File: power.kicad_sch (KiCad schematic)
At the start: 10 parts, among them U19 SN74ALS04 (КР1533ЛН1), U21 SN74ALS14 (КР1533ТЛ2), U39 IN74ALS32N (КР1533ЛЛ1), U40 IN74ALS00N (КР1533ЛА3), U75 IN74ALS32N (КР1533ЛЛ1)

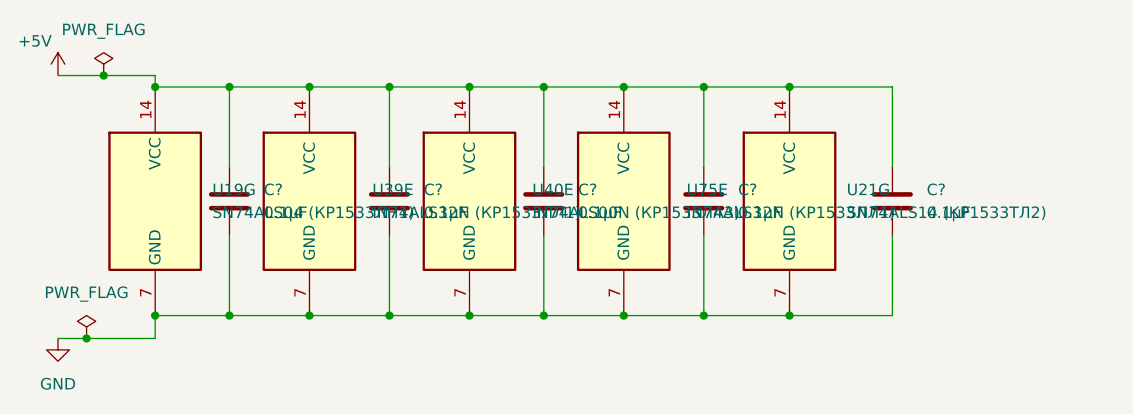
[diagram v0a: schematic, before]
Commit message: March 22nd additions
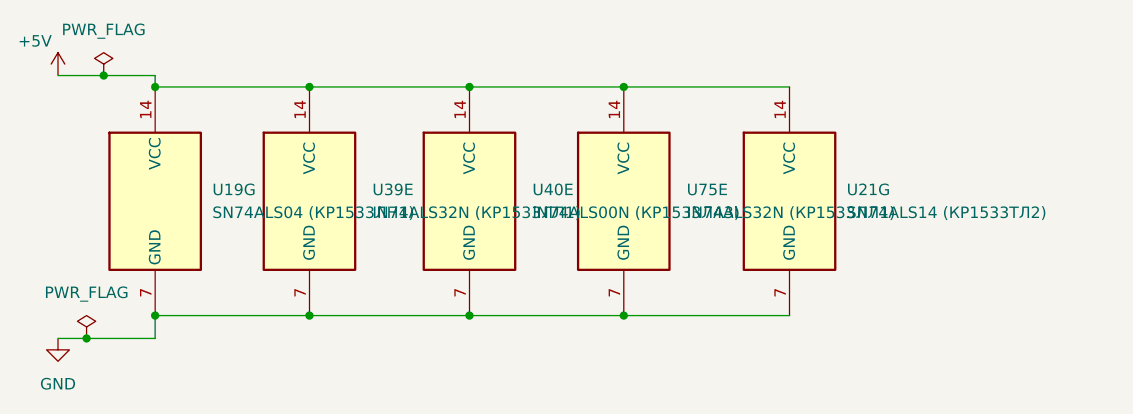
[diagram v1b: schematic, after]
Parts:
- removed C? (x5): 0.1µF, Capacitor_SMD:C_0805_2012Metric, symbol Device:C
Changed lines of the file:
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@@
     (comment 2 "Евстафьев")
   )
-  (junction (at 80.645 54.61) (diameter 0) (color 0 0 0 0)
-  )
-  (junction (at 98.425 54.61) (diameter 0) (color 0 0 0 0)
-  )
-  (junction (at 45.72 29.21) (diameter 0) (color 0 0 0 0)
-  )
   (junction (at 72.39 54.61) (diameter 0) (color 0 0 0 0)
   )
   (junction (at 37.465 29.21) (diameter 0) (color 0 0 0 0)
   )
-  (junction (at 45.72 54.61) (diameter 0) (color 0 0 0 0)
-  )
-  (junction (at 107.95 54.61) (diameter 0) (color 0 0 0 0)
-  )
   (junction (at 29.845 57.15) (diameter 0) (color 0 0 0 0)
   )
@@
   (junction (at 54.61 29.21) (diameter 0) (color 0 0 0 0)
   )
-  (junction (at 98.425 29.21) (diameter 0) (color 0 0 0 0)
-  )
-  (junction (at 107.95 29.21) (diameter 0) (color 0 0 0 0)
-  )
   (junction (at 31.75 27.94) (diameter 0) (color 0 0 0 0)
   )
-  (junction (at 63.5 54.61) (diameter 0) (color 0 0 0 0)
-  )
   (junction (at 72.39 29.21) (diameter 0) (color 0 0 0 0)
   )
-  (junction (at 63.5 29.21) (diameter 0) (color 0 0 0 0)
-  )
-  (junction (at 80.645 29.21) (diameter 0) (color 0 0 0 0)
-  )
   (junction (at 89.535 29.21) (diameter 0) (color 0 0 0 0)
   )
   (junction (at 37.465 54.61) (diameter 0) (color 0 0 0 0)
   )
-  (wire (pts (xy 98.425 29.21) (xy 107.95 29.21))
-    (stroke (width 0) (type default) (color 0 0 0 0))
-  )
-  (wire (pts (xy 119.38 45.72) (xy 119.38 54.61))
-    (stroke (width 0) (type default) (color 0 0 0 0))
-  )
-  (wire (pts (xy 119.38 38.1) (xy 119.38 29.21))
-    (stroke (width 0) (type default) (color 0 0 0 0))
-  )
-  (wire (pts (xy 98.425 54.61) (xy 89.535 54.61))
-    (stroke (width 0) (type default) (color 0 0 0 0))
-  )
-  (wire (pts (xy 45.72 29.21) (xy 54.61 29.21))
-    (stroke (width 0) (type default) (color 0 0 0 0))
-  )
-  (wire (pts (xy 63.5 38.1) (xy 63.5 29.21))
-    (stroke (width 0) (type default) (color 0 0 0 0))
-  )
-  (wire (pts (xy 37.465 29.21) (xy 45.72 29.21))
-    (stroke (width 0) (type default) (color 0 0 0 0))
-  )
-  (wire (pts (xy 119.38 29.21) (xy 107.95 29.21))
+  (wire (pts (xy 89.535 29.21) (xy 107.95 29.21))
+    (stroke (width 0) (type default) (color 0 0 0 0))
+  )
+  (wire (pts (xy 89.535 54.61) (xy 107.95 54.61))
+    (stroke (width 0) (type default) (color 0 0 0 0))
+  )
+  (wire (pts (xy 37.465 29.21) (xy 54.61 29.21))
     (stroke (width 0) (type default) (color 0 0 0 0))
   )
@@
     (stroke (width 0) (type default) (color 0 0 0 0))
   )
-  (wire (pts (xy 80.645 45.72) (xy 80.645 54.61))
-    (stroke (width 0) (type default) (color 0 0 0 0))
-  )
   (wire (pts (xy 26.67 27.94) (xy 31.75 27.94))
     (stroke (width 0) (type default) (color 0 0 0 0))
   )
-  (wire (pts (xy 54.61 29.21) (xy 63.5 29.21))
-    (stroke (width 0) (type default) (color 0 0 0 0))
-  )
-  (wire (pts (xy 119.38 54.61) (xy 107.95 54.61))
-    (stroke (width 0) (type default) (color 0 0 0 0))
-  )
   (wire (pts (xy 31.75 27.94) (xy 37.465 27.94))
     (stroke (width 0) (type default) (color 0 0 0 0))
   )
-  (wire (pts (xy 45.72 54.61) (xy 54.61 54.61))
+  (wire (pts (xy 37.465 54.61) (xy 54.61 54.61))
     (stroke (width 0) (type default) (color 0 0 0 0))
   )
@@
     (stroke (width 0) (type default) (color 0 0 0 0))
   )
-  (wire (pts (xy 37.465 54.61) (xy 45.72 54.61))
-    (stroke (width 0) (type default) (color 0 0 0 0))
-  )
-  (wire (pts (xy 80.645 54.61) (xy 89.535 54.61))
-    (stroke (width 0) (type default) (color 0 0 0 0))
-  )
-  (wire (pts (xy 54.61 54.61) (xy 63.5 54.61))
-    (stroke (width 0) (type default) (color 0 0 0 0))
-  )
-  (wire (pts (xy 45.72 29.21) (xy 45.72 38.1))
-    (stroke (width 0) (type default) (color 0 0 0 0))
-  )
-  (wire (pts (xy 63.5 45.72) (xy 63.5 54.61))
-    (stroke (width 0) (type default) (color 0 0 0 0))
-  )
-  (wire (pts (xy 63.5 54.61) (xy 72.39 54.61))
-    (stroke (width 0) (type default) (color 0 0 0 0))
-  )
-  (wire (pts (xy 98.425 45.72) (xy 98.425 54.61))
-    (stroke (width 0) (type default) (color 0 0 0 0))
-  )
-  (wire (pts (xy 45.72 45.72) (xy 45.72 54.61))
-    (stroke (width 0) (type default) (color 0 0 0 0))
-  )
-  (wire (pts (xy 80.645 29.21) (xy 80.645 38.1))
-    (stroke (width 0) (type default) (color 0 0 0 0))
-  )
-  (wire (pts (xy 80.645 29.21) (xy 89.535 29.21))
-    (stroke (width 0) (type default) (color 0 0 0 0))
-  )
-  (wire (pts (xy 107.95 54.61) (xy 98.425 54.61))
-    (stroke (width 0) (type default) (color 0 0 0 0))
-  )
-  (wire (pts (xy 98.425 29.21) (xy 89.535 29.21))
+  (wire (pts (xy 54.61 54.61) (xy 72.39 54.61))
     (stroke (width 0) (type default) (color 0 0 0 0))
   )
@@
     (stroke (width 0) (type default) (color 0 0 0 0))
   )
-  (wire (pts (xy 63.5 29.21) (xy 72.39 29.21))
-    (stroke (width 0) (type default) (color 0 0 0 0))
-  )
-  (wire (pts (xy 98.425 38.1) (xy 98.425 29.21))
-    (stroke (width 0) (type default) (color 0 0 0 0))
-  )
-  (wire (pts (xy 72.39 54.61) (xy 80.645 54.61))
+  (wire (pts (xy 54.61 29.21) (xy 72.39 29.21))
+    (stroke (width 0) (type default) (color 0 0 0 0))
+  )
+  (wire (pts (xy 72.39 54.61) (xy 89.535 54.61))
     (stroke (width 0) (type default) (color 0 0 0 0))
   )
@@
     (stroke (width 0) (type default) (color 0 0 0 0))
   )
-  (wire (pts (xy 72.39 29.21) (xy 80.645 29.21))
+  (wire (pts (xy 72.39 29.21) (xy 89.535 29.21))
     (stroke (width 0) (type default) (color 0 0 0 0))
   )
@@
     )
     (pin "1")
-  )
-  (symbol (lib_id "Device:C") (at 119.38 41.91 0) (unit 1)
-    (in_bom yes) (on_board yes) (fields_autoplaced)
-    (property "Reference" "C?" (id 0) (at 123.19 40.6399 0)
-      (effects (font (size 1.27 1.27)) (justify left))
-    )
-    (property "Value" "0.1µF" (id 1) (at 123.19 43.1799 0)
-      (effects (font (size 1.27 1.27)) (justify left))
-    )
-    (property "Footprint" "Capacitor_SMD:C_0805_2012Metric" (id 2) (at 120.3452 45.72 0)
-      (effects (font (size 1.27 1.27)) hide)
-    )
-    (property "Datasheet" "~" (id 3) (at 119.38 41.91 0)
-      (effects (font (size 1.27 1.27)) hide)
-    )
-    (pin "1")
-    (pin "2")
   )
   (symbol (lib_id "74xx:74LS14") (at 107.95 41.91 0) (unit 7)
@@
     (pin "1")
   )
-  (symbol (lib_id "Device:C") (at 45.72 41.91 0) (unit 1)
-    (in_bom yes) (on_board yes) (fields_autoplaced)
-    (property "Reference" "C?" (id 0) (at 49.53 40.6399 0)
-      (effects (font (size 1.27 1.27)) (justify left))
-    )
-    (property "Value" "0.1µF" (id 1) (at 49.53 43.1799 0)
-      (effects (font (size 1.27 1.27)) (justify left))
-    )
-    (property "Footprint" "Capacitor_SMD:C_0805_2012Metric" (id 2) (at 46.6852 45.72 0)
-      (effects (font (size 1.27 1.27)) hide)
-    )
-    (property "Datasheet" "~" (id 3) (at 45.72 41.91 0)
-      (effects (font (size 1.27 1.27)) hide)
-    )
-    (pin "1")
-    (pin "2")
-  )
-  (symbol (lib_id "Device:C") (at 80.645 41.91 0) (unit 1)
-    (in_bom yes) (on_board yes) (fields_autoplaced)
-    (property "Reference" "C?" (id 0) (at 84.455 40.6399 0)
-      (effects (font (size 1.27 1.27)) (justify left))
-    )
-    (property "Value" "0.1µF" (id 1) (at 84.455 43.1799 0)
-      (effects (font (size 1.27 1.27)) (justify left))
-    )
-    (property "Footprint" "Capacitor_SMD:C_0805_2012Metric" (id 2) (at 81.6102 45.72 0)
-      (effects (font (size 1.27 1.27)) hide)
-    )
-    (property "Datasheet" "~" (id 3) (at 80.645 41.91 0)
-      (effects (font (size 1.27 1.27)) hide)
-    )
-    (pin "1")
-    (pin "2")
-  )
-  (symbol (lib_id "Device:C") (at 63.5 41.91 0) (unit 1)
-    (in_bom yes) (on_board yes) (fields_autoplaced)
-    (property "Reference" "C?" (id 0) (at 67.31 40.6399 0)
-      (effects (font (size 1.27 1.27)) (justify left))
-    )
-    (property "Value" "0.1µF" (id 1) (at 67.31 43.1799 0)
-      (effects (font (size 1.27 1.27)) (justify left))
-    )
-    (property "Footprint" "Capacitor_SMD:C_0805_2012Metric" (id 2) (at 64.4652 45.72 0)
-      (effects (font (size 1.27 1.27)) hide)
-    )
-    (property "Datasheet" "~" (id 3) (at 63.5 41.91 0)
-      (effects (font (size 1.27 1.27)) hide)
-    )
-    (pin "1")
-    (pin "2")
-  )
-  (symbol (lib_id "Device:C") (at 98.425 41.91 0) (unit 1)
-    (in_bom yes) (on_board yes) (fields_autoplaced)
-    (property "Reference" "C?" (id 0) (at 102.235 40.6399 0)
-      (effects (font (size 1.27 1.27)) (justify left))
-    )
-    (property "Value" "0.1µF" (id 1) (at 102.235 43.1799 0)
-      (effects (font (size 1.27 1.27)) (justify left))
-    )
-    (property "Footprint" "Capacitor_SMD:C_0805_2012Metric" (id 2) (at 99.3902 45.72 0)
-      (effects (font (size 1.27 1.27)) hide)
-    )
-    (property "Datasheet" "~" (id 3) (at 98.425 41.91 0)
-      (effects (font (size 1.27 1.27)) hide)
-    )
-    (pin "1")
-    (pin "2")
-  )
 )
